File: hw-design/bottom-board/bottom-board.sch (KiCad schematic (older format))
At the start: 0 parts

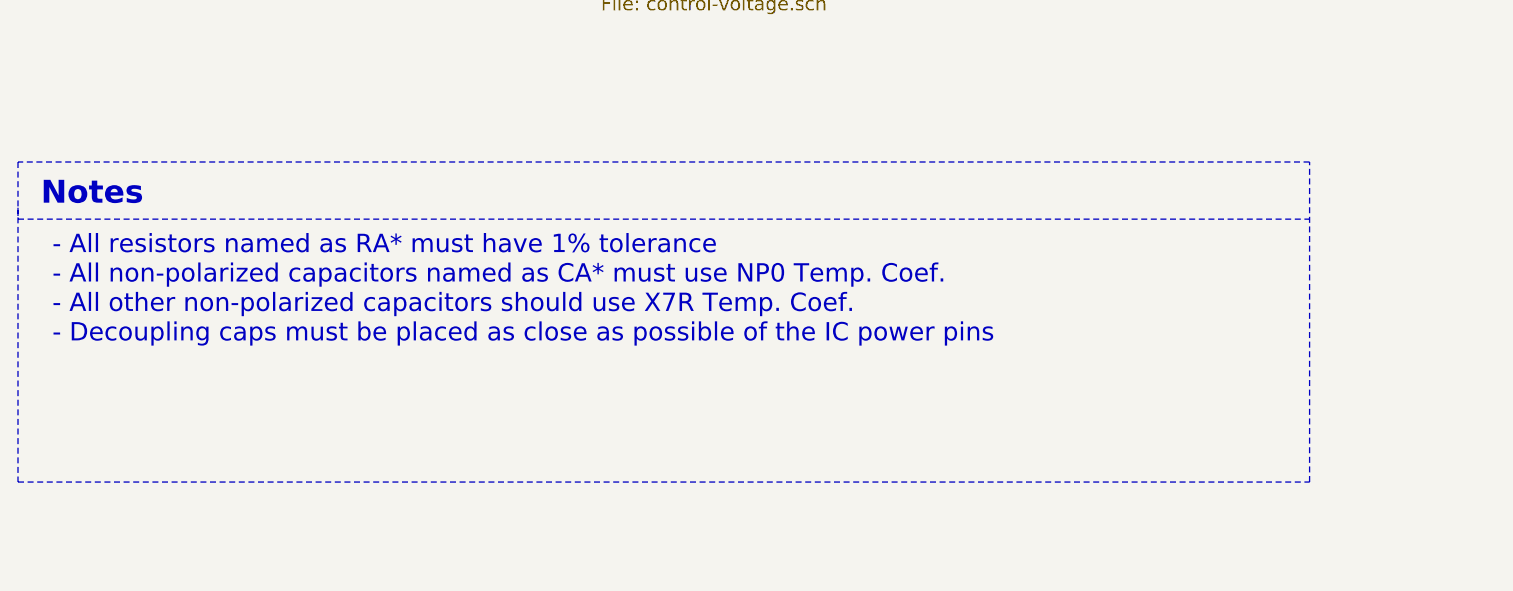
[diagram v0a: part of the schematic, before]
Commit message: bottom,sch: minor adjustments
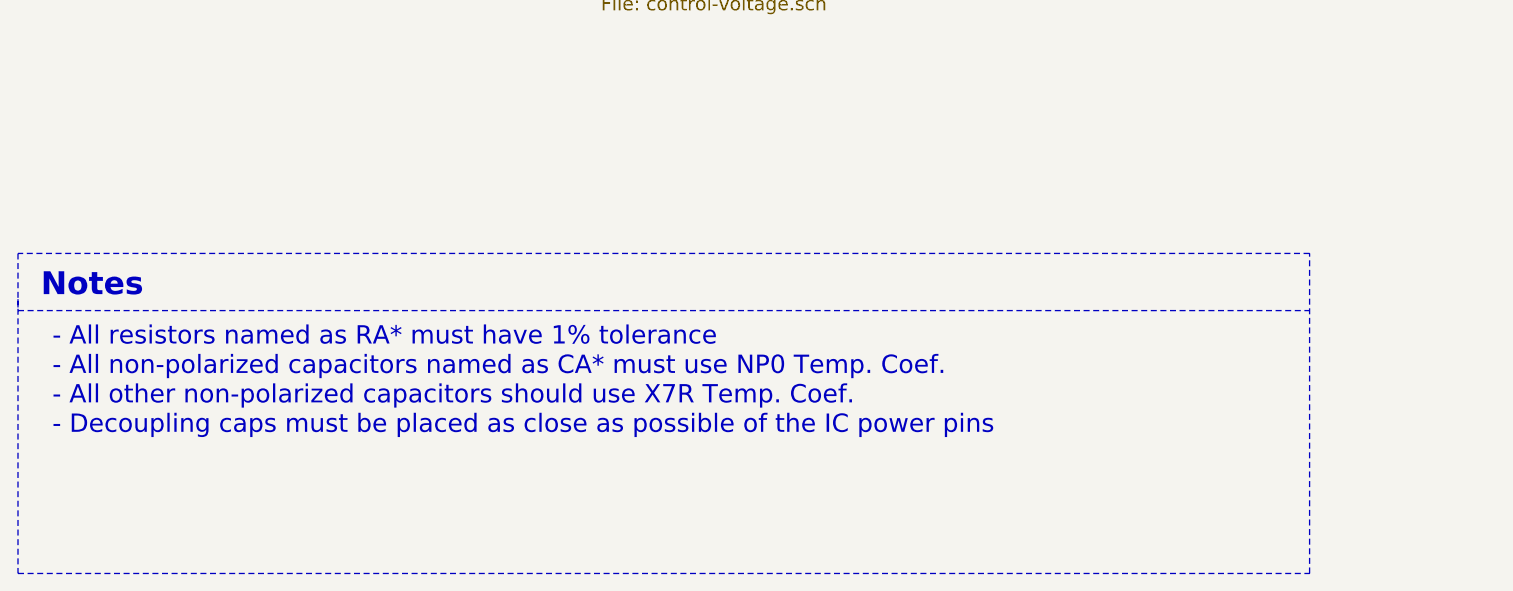
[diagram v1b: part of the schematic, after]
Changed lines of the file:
@@
 F1 "connectors.sch" 60
 $EndSheet
-Text Notes 1350 5600 0    80   ~ 0
+Text Notes 1350 6000 0    80   ~ 0
 - All resistors named as RA* must have 1% tolerance\n- All non-polarized capacitors named as CA* must use NP0 Temp. Coef.\n- All other non-polarized capacitors should use X7R Temp. Coef.\n- Decoupling caps must be placed as close as possible of the IC power pins
-Text Notes 1300 5000 0    100  ~ 20
+Text Notes 1300 5400 0    100  ~ 20
 Notes\n
 Wire Notes Line
-	1200 5000 1200 6200
+	1200 5400 1200 6600
 Wire Notes Line
-	1200 6200 6850 6200
+	1200 6600 6850 6600
 Wire Notes Line
-	6850 6200 6850 4800
+	6850 6600 6850 5200
 Wire Notes Line
-	6850 4800 1200 4800
+	6850 5200 1200 5200
 Wire Notes Line
-	1200 4800 1200 5050
+	1200 5200 1200 5450
 Wire Notes Line
-	1200 5050 6850 5050
+	1200 5450 6850 5450
 $Sheet
 S 1300 2250 2150 400
